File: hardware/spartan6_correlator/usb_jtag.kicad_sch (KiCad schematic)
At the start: 4 parts, among them J1 JST_SHL_SM08B, J2 USB_C_Receptacle_USB2.0_16P, U6 FT2232D, U7 93LCxxB

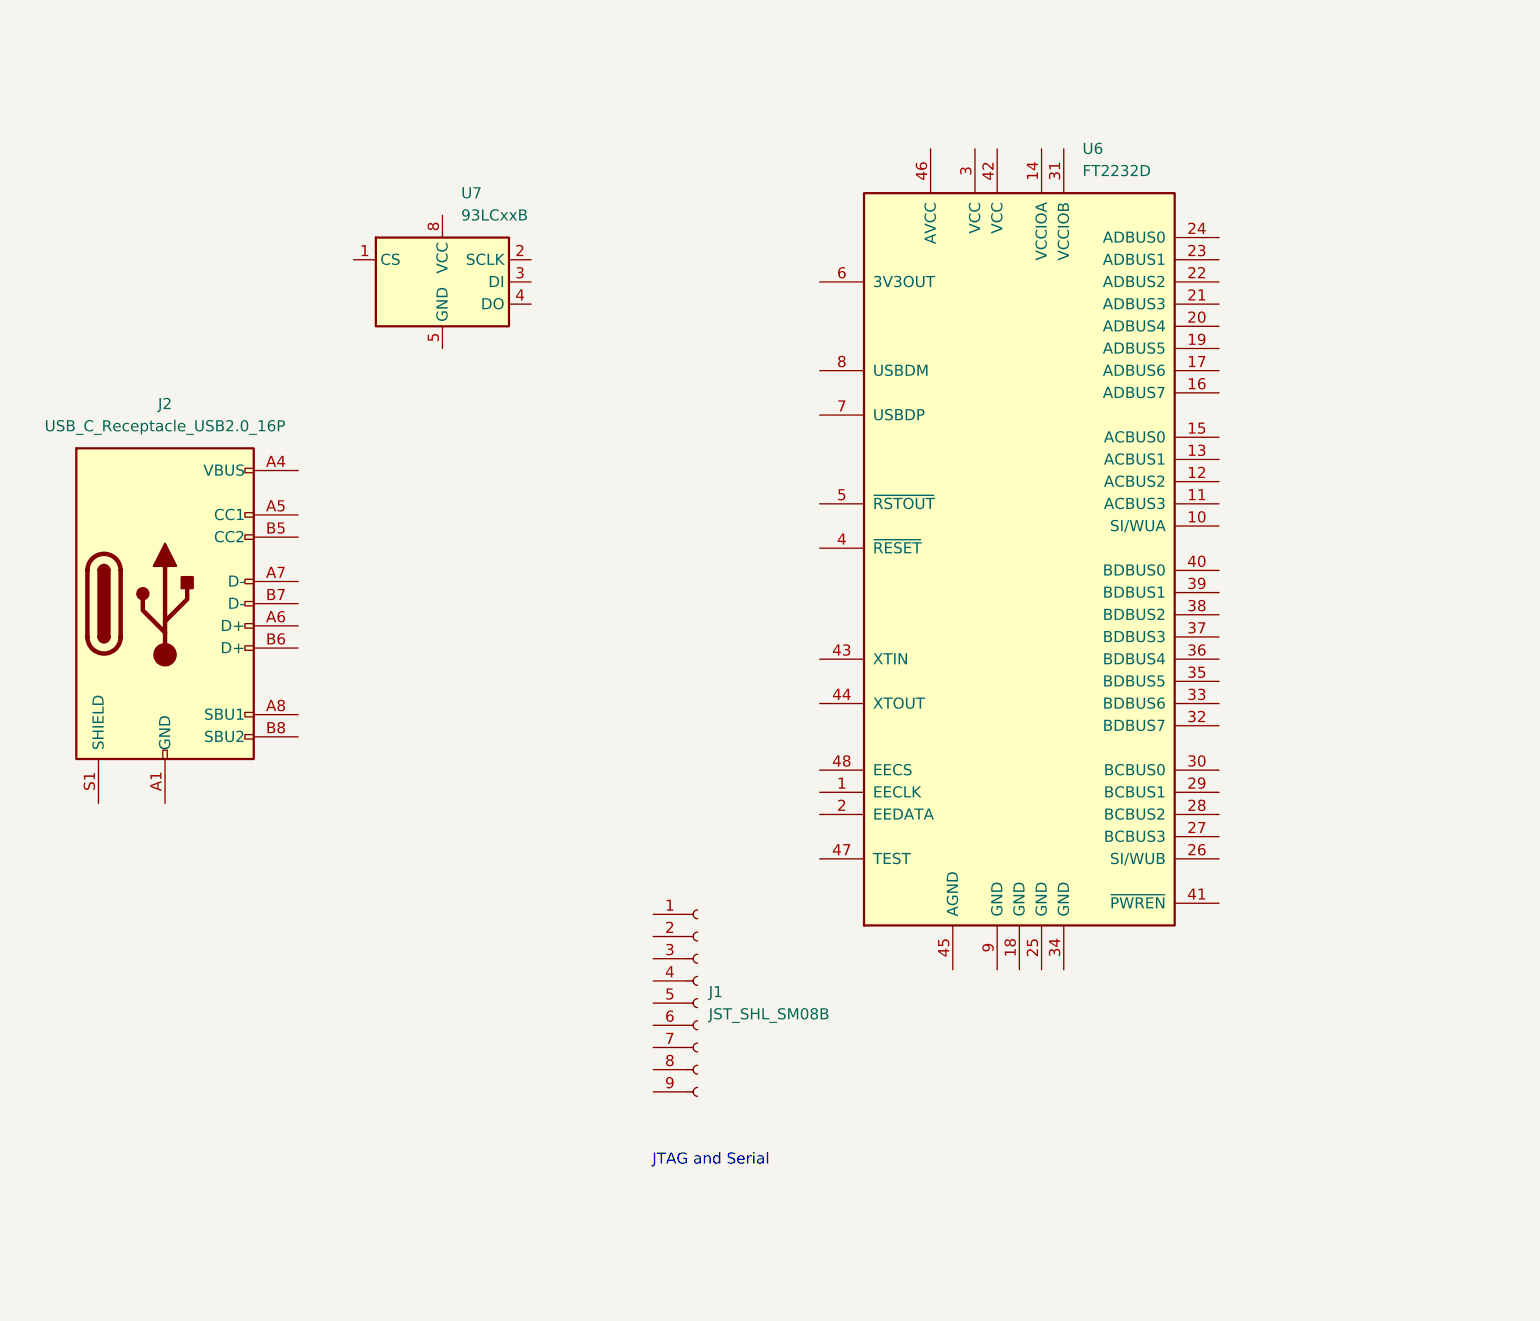
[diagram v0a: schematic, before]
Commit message: Updates. Lots of them
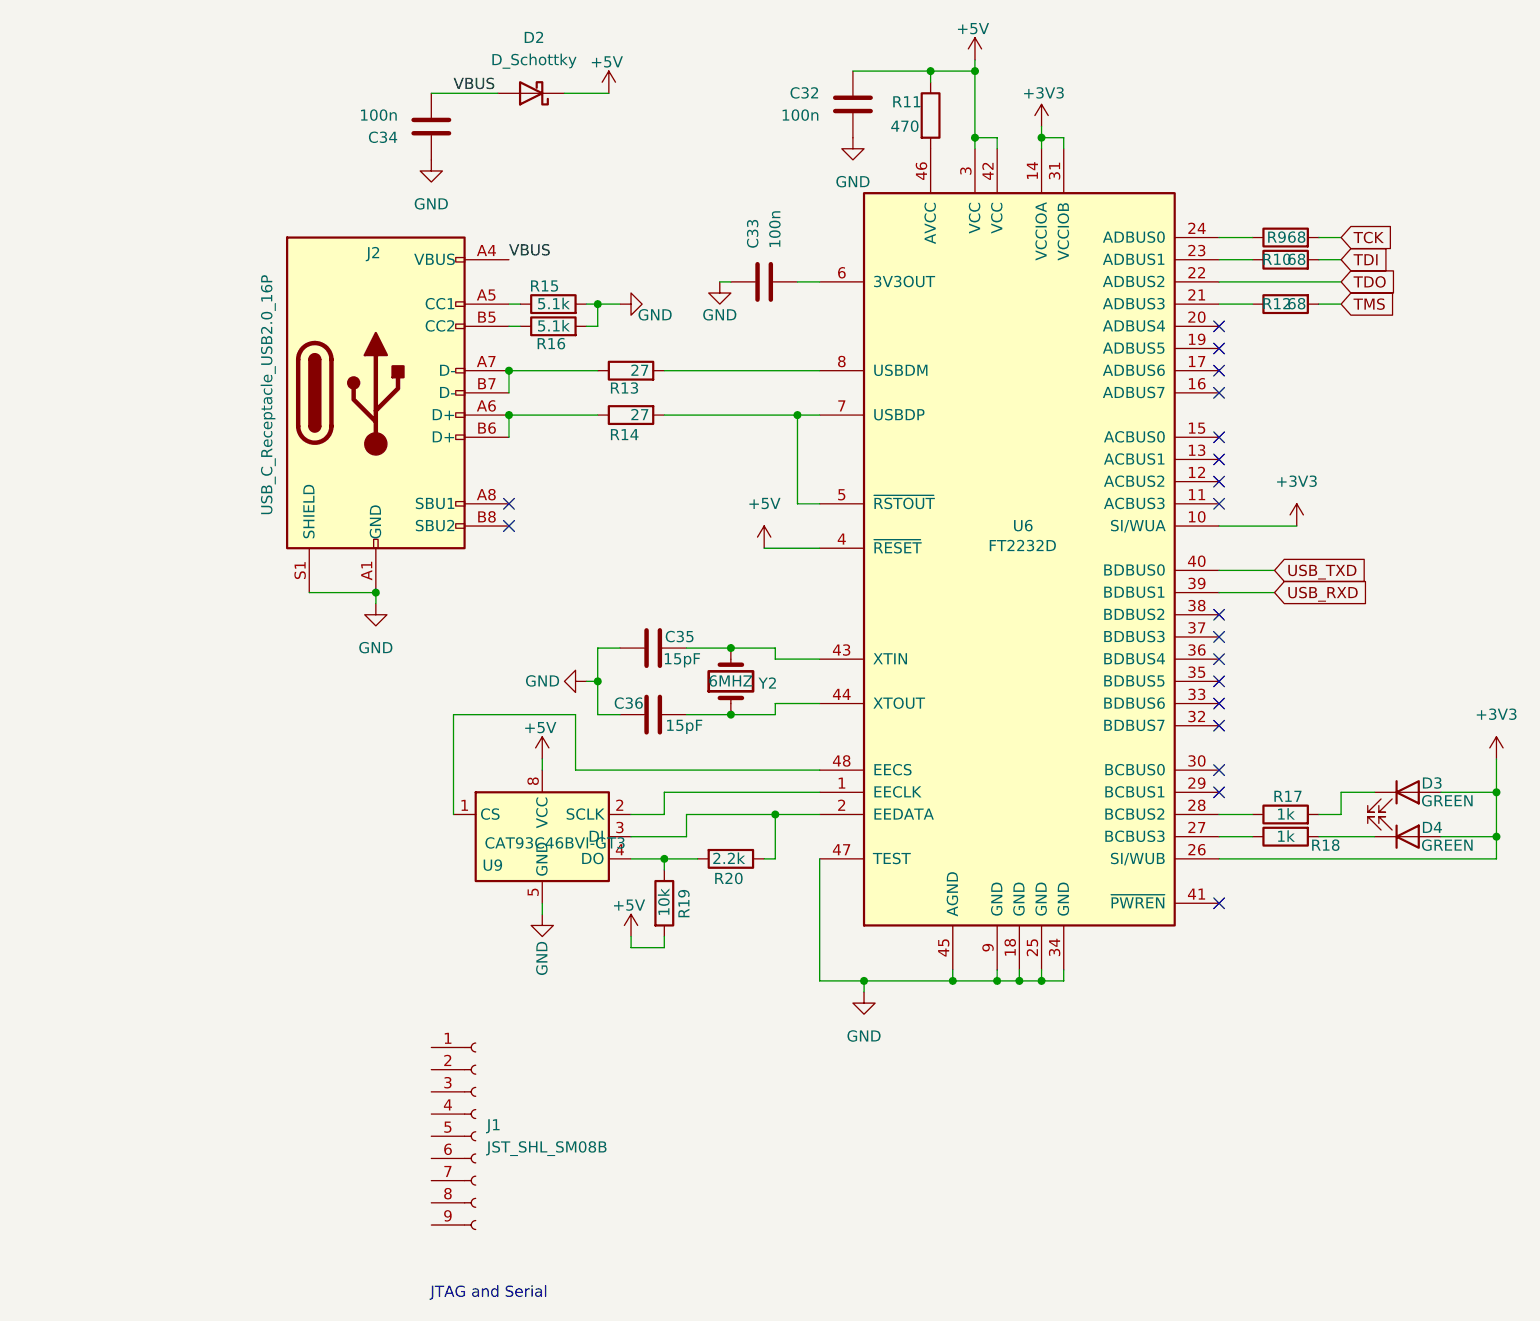
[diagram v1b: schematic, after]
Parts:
- removed U7: 93LCxxB, symbol Memory_EEPROM:93LCxxB
- added C32, C33, C34: 100n, symbol Device:C
- added C35, C36: 15pF, symbol Device:C
- added D2: D_Schottky, Diode_SMD:D_SMA, symbol Device:D_Schottky
- added D3, D4: GREEN, symbol Device:LED
- added R10, R12, R9: 68, symbol Device:R
- added R11: 470, symbol Device:R
- added R13, R14: 27, symbol Device:R
- added R15, R16: 5.1k, symbol Device:R
- added R17, R18: 1k, symbol Device:R
- added R19: 10k, symbol Device:R
- added R20: 2.2k, symbol Device:R
- added U9: CAT93C46BVI-GT3, Package_SO:SOIC-8_3.9x4.9mm_P1.27mm, symbol Memory_EEPROM:93CxxB
- added Y2: 6MHZ, Crystal:Crystal_SMD_3225-4Pin_3.2x2.5mm, symbol Device:Crystal
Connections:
- net GND: now reaches J2.A1 (GND), J2.A12 (GND), J2.B1 (GND), J2.B12 (GND)
- net GND: now also J2.S1 (SHIELD), U6.18 (GND), U6.25 (GND), U6.34 (GND), U6.45 (AGND), U6.47 (TEST), U6.9 (GND), C32.2, C33.1, C34.1, C35.1, C36.1, R15.2, R16.2, U9.5 (GND)
- net VBUS: now reaches J2.A4 (VBUS), J2.A9 (VBUS), J2.B4 (VBUS), J2.B9 (VBUS)
- net VBUS: now also C34.2, D2.2 (A)
- net at J2.A5 (CC1): now also R15.1
- net at J2.A6 (D+): now also J2.B6 (D+), R14.1
- net at J2.A7 (D-): now also J2.B7 (D-), R13.1
- net at J2.B5 (CC2): now also R16.1
- net at U6.1 (EECLK): now also U9.2 (SCLK)
- net +3V3: now reaches U6.10 (SI/WUA)
- net +3V3: now also U6.14 (VCCIOA), U6.26 (SI/WUB), U6.31 (VCCIOB), D3.2 (A), D4.2 (A)
- net at U6.2 (EEDATA): now also R20.1, U9.3 (DI)
- net at U6.21 (ADBUS3): now also R12.1
- net TDO: now reaches U6.22 (ADBUS2)
- net at U6.23 (ADBUS1): now also R10.1
- net at U6.24 (ADBUS0): now also R9.1
- net at U6.27 (BCBUS3): now also R18.1
- net at U6.28 (BCBUS2): now also R17.1
- net +5V: now reaches U6.3 (VCC)
- net +5V: now also U6.4 (~{RESET}), U6.42 (VCC), C32.1, D2.1 (K), R11.1, R19.2, U9.8 (VCC)
- net USB_RXD: now reaches U6.39 (BDBUS1)
- net USB_TXD: now reaches U6.40 (BDBUS0)
- net at U6.43 (XTIN): now also C35.2, Y2.2
- net at U6.44 (XTOUT): now also C36.2, Y2.1
- net at U6.46 (AVCC): now also R11.2
- net at U6.48 (EECS): now also U9.1 (CS)
- net at U6.5 (~{RSTOUT}): now also U6.7 (USBDP), R14.2
- net at U6.6 (3V3OUT): now also C33.2
- net at U6.8 (USBDM): now also R13.2
- new net: D4.1 (K), R18.2
- new net: R19.1, R20.2, U9.4 (DO)
- new net: D3.1 (K), R17.2
- new net TCK: R9.2
- new net TDI: R10.2
- new net TMS: R12.2
- no-connect marks 0 -> 19
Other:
- moved on the sheet: J1, J2
